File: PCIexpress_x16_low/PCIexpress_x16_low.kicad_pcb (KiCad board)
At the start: 4 copper layers, 312 x 111.2 mm, 66 parts, among them J1 PCIexpress_bracket, J2 PCIexpress_x16

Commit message: templates
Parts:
- J1: footprint PCIexpress:PCIexpress_bracket_full -> PCIexpress:PCIexpress_bracket_low
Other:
- board size 312 x 111.2 mm -> 167.7 x 68.9 mm

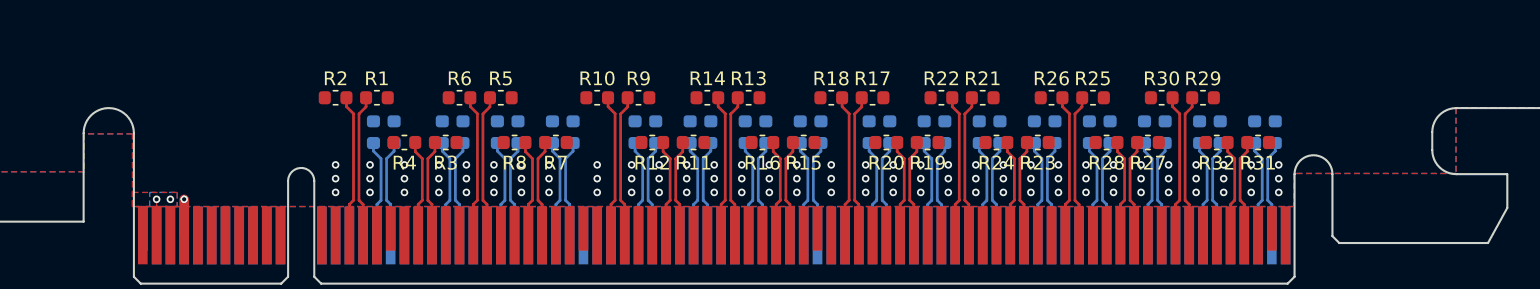
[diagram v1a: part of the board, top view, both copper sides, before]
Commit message: KiCad 6 update
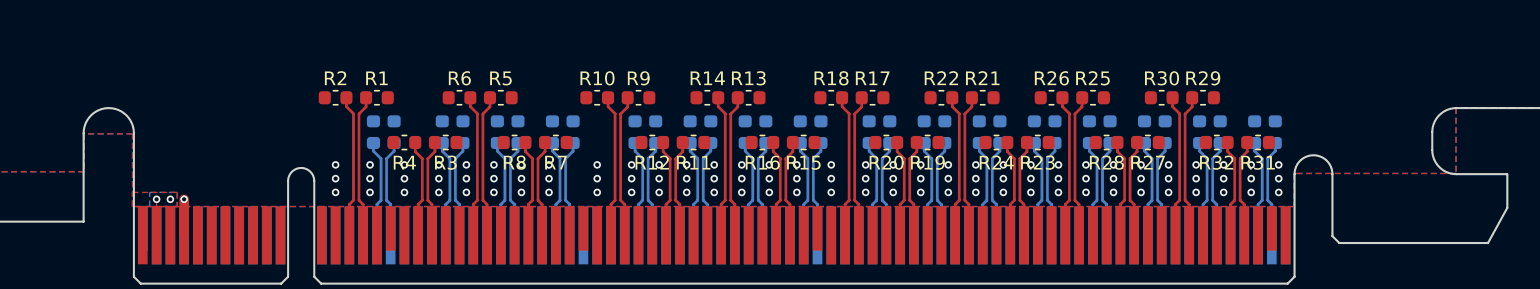
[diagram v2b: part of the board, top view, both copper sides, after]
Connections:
- net /~PERST renamed /~{PERST}
- net /~PRSNT1 renamed /~{PRSNT1}
- net /~PRSNT2x1 renamed /~{PRSNT2x1}
- net /~PRSNT2x16 renamed /~{PRSNT2x16}
- net /~PRSNT2x4 renamed /~{PRSNT2x4}
- net /~PRSNT2x8 renamed /~{PRSNT2x8}
- net /~TRST renamed /~{TRST}
- net /~WAKE renamed /~{WAKE}
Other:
- net class Default removed
- net class Diff-100-PCIe removed
- net class JLC2313-100d-3.5 removed
- net class JLC2313-100d-4 removed
- net class JLC7628-100d-8 removed
